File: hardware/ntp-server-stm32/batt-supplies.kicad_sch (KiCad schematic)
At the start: 24 parts, among them U34 TPS61094DSSR, U35 TPS61094DSSR

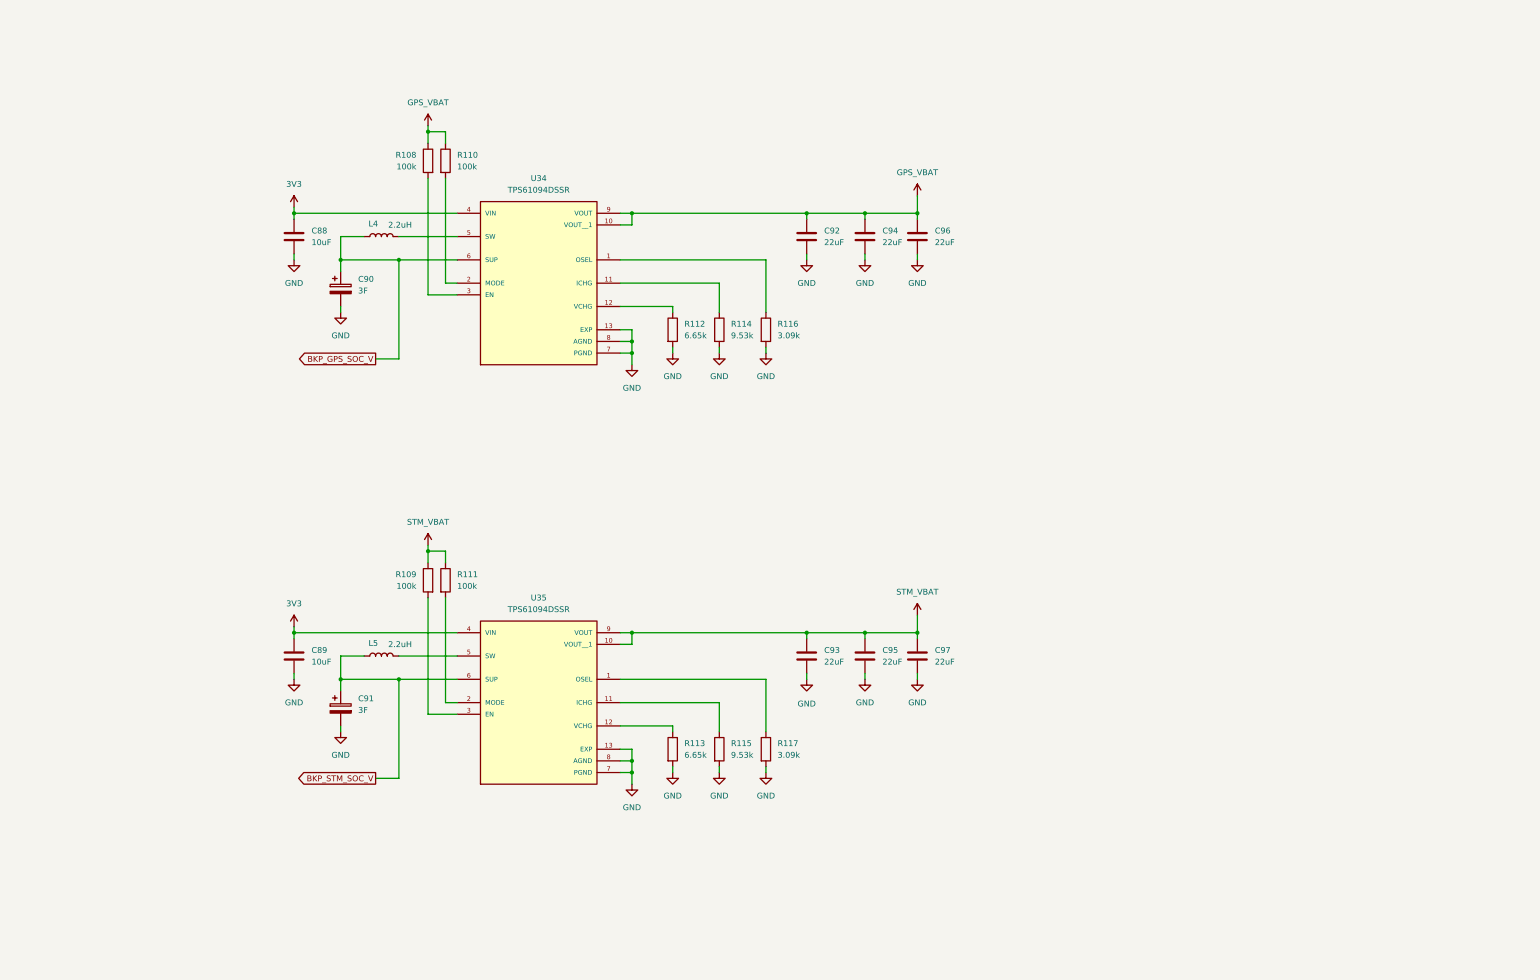
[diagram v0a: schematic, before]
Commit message: Updates
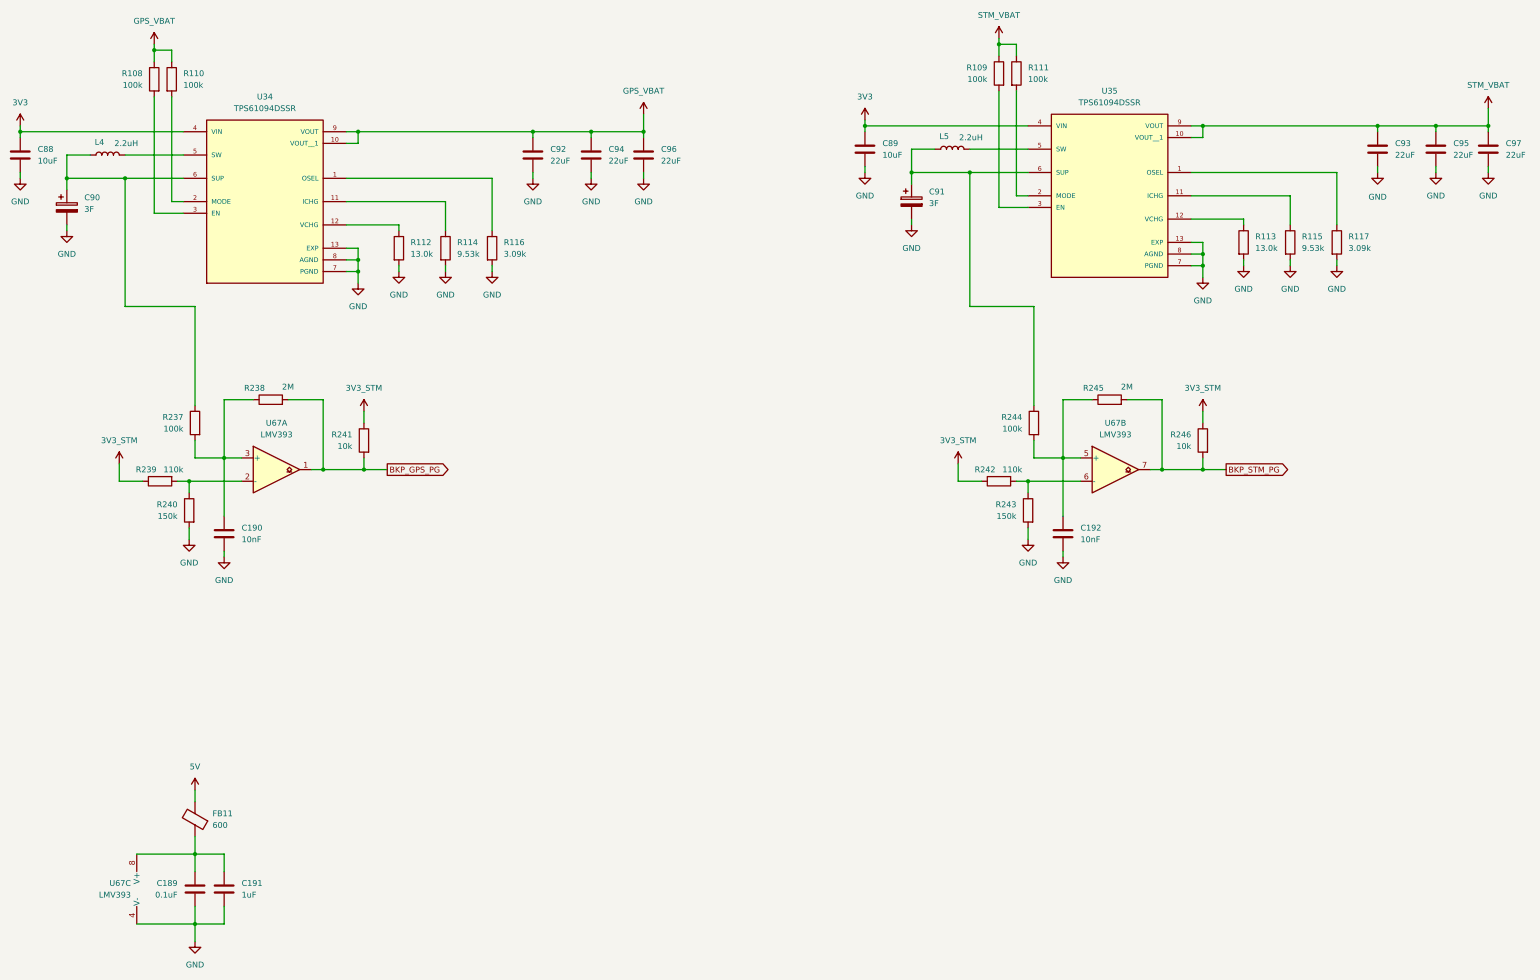
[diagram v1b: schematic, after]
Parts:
- added C189: 0.1uF, 0402 (1005 Metric), symbol Device:C
- added C190, C192: 10nF, 0402 (1005 Metric), symbol Device:C
- added C191: 1uF, 0603 (1608 Metric), symbol Device:C
- added FB11: 600, 1206, symbol Device:FerriteBead
- added R237, R244: 100k, 0402 (1005 Metric), symbol Device:R
- added R238, R245: 2M, 0402 (1005 Metric), symbol Device:R
- added R239, R242: 110k, R_0402_1005Metric, symbol Device:R
- added R240, R243: 150k, R_0402_1005Metric, symbol Device:R
- added R241, R246: 10k, 0402 (1005 Metric), symbol Device:R
- added U67: LMV393, symbol Comparator:LMV393
- C88, C89: footprint C_0805_2012Metric -> 1206 (3216 Metric); DIELECTRIC (none) -> X7R; DIGIKEY_PART_NUMBER 490-GRM21BZ71C106KE15LTR-ND -> 1276-6797-1-ND; MANUFACTURER Murata -> Samsung Electro-Mechanics; MANUFACTURER_PART_NUMBER GRM21BZ71C106KE15L -> CL31B106KOHVPNE; TOLERANCE (none) -> 10%; VOLTAGE (none) -> 16V
- C90, C91: DIELECTRIC (none) -> EDLC; MANUFACTURER Cornell Dubilier Knowles -> Cornell Dubilier; TOLERANCE (none) -> 5%; VOLTAGE (none) -> 3V
- C92, C93, C94, C95, C96, C97: footprint C_0805_2012Metric -> 0805 (2012 Metric); DIELECTRIC (none) -> X5R; DIGIKEY_PART_NUMBER (none) -> 490-GRT21BR61C226ME13KCT-ND; MANUFACTURER (none) -> Murata Electronics; MANUFACTURER_PART_NUMBER (none) -> GRT21BR61C226ME13K; TOLERANCE (none) -> 10%; VOLTAGE (none) -> 16V
- L4, L5: DIELECTRIC (none) -> Inductor
- R108, R109, R110, R111: footprint R_0402_1005Metric -> 0402 (1005 Metric); DIELECTRIC (none) -> Thick-film; DIGIKEY_PART_NUMBER (none) -> P100KLCT-ND; MANUFACTURER Panasonic -> Panasonic Industry; POWER (none) -> 1/10W; TOLERANCE (none) -> 1%
- R112, R113: value 6.65k -> 13.0k; footprint R_0402_1005Metric -> 0402 (1005 Metric); DIELECTRIC (none) -> Thick-film; DIGIKEY_PART_NUMBER (none) -> P13.0KLCT-ND; MANUFACTURER Panasonic -> Panasonic Industry; MANUFACTURER_PART_NUMBER ERJ-2RKF6651X -> ERJ-2RKF1302X; POWER (none) -> 1/10W; TOLERANCE (none) -> 1%
- R114, R115: footprint R_0402_1005Metric -> 0402 (1005 Metric); DIELECTRIC (none) -> Thick-film; DIGIKEY_PART_NUMBER (none) -> P9.53KLCT-ND; MANUFACTURER Panasonic -> Panasonic Industry; POWER (none) -> 1/10W; TOLERANCE (none) -> 1%
- R116, R117: footprint R_0402_1005Metric -> 0402 (1005 Metric); DIELECTRIC (none) -> Thick-film; DIGIKEY_PART_NUMBER (none) -> P3.09KLCT-ND; MANUFACTURER Panasonic -> Panasonic Industry; POWER (none) -> 1/10W; TOLERANCE (none) -> 1%
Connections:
- net GND: now also C189.2, C190.2, C191.2, C192.2, R240.2, R243.2, U67.4 (V-)
- net BKP_GPS_SOC_V: no longer names the net of C90.1, L4.2, U34.6 (SUP)
- net BKP_GPS_SOC_V: now also R237.1
- net BKP_STM_SOC_V: no longer names the net of C91.1, L5.2, U35.6 (SUP)
- net BKP_STM_SOC_V: now also R244.1
- new net: C190.1, R237.2, R238.1, U67.3 (+)
- new net: R239.2, R240.1, U67.2 (-)
- new net: R242.2, R243.1, U67.6 (-)
- new net: C192.1, R244.2, R245.1, U67.5 (+)
- new net: C189.1, C191.1, FB11.1, U67.8 (V+)
- new net 3V3_STM: R239.1, R241.1, R242.1, R246.1
- new net 5V: FB11.2
- new net BKP_GPS_PG: R238.2, R241.2, U67.1
- new net BKP_STM_PG: R245.2, R246.2, U67.7
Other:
- moved on the sheet: C88, C89, C90, C91, C92, C93, C94, C95, C96, C97, L4, L5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

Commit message: Bom updates
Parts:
- FB11: footprint 1206 -> 1206 (3216 Metric)
- L4, L5: DIGIKEY_PART_NUMBER (none) -> 283-DR73-2R2-RTR-ND; MANUFACTURER (none) -> Eaton - Electronics Division; MANUFACTURER_PART_NUMBER (none) -> DR73-2R2-R
- R239, R242: footprint R_0402_1005Metric -> 0402 (1005 Metric); DIGIKEY_PART_NUMBER (none) -> P110KLCT-ND; MANUFACTURER Panasonic -> Panasonic Industry
- R240, R243: footprint R_0402_1005Metric -> 0402 (1005 Metric); DIGIKEY_PART_NUMBER (none) -> P150KLCT-ND; MANUFACTURER Panasonic -> Panasonic Industry
- U34, U35: DIGIKEY_PART_NUMBER (none) -> 296-TPS61094DSSRCT-ND
- U67: footprint (none) -> 8-VSSOP; DIGIKEY_PART_NUMBER (none) -> 296-13993-1-ND
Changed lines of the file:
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@@
 			)
 		)
-		(property "Footprint" "R_0402_1005Metric"
+		(property "Footprint" "0402 (1005 Metric)"
 			(at 69.85 126.492 90)
 			(hide yes)
@@
 			)
 		)
-		(property "Datasheet" ""
+		(property "Datasheet" "https://industrial.panasonic.com/cdbs/www-data/pdf/RDA0000/AOA0000C304.pdf"
 			(at 69.85 128.27 0)
 			(hide yes)
@@
 			)
 		)
-		(property "Description" "RES 110k 1% 1/10W 0402"
+		(property "Description" "RES SMD 110K OHM 1% 1/10W 0402"
 			(at 69.85 128.27 0)
 			(hide yes)
@@
 			)
 		)
-		(property "MANUFACTURER" "Panasonic"
+		(property "MANUFACTURER" "Panasonic Industry"
 			(at 11.43 256.54 0)
 			(hide yes)
@@
 			)
 		)
+		(property "DIGIKEY_PART_NUMBER" "P110KLCT-ND"
+			(at 69.85 128.27 90)
+			(hide yes)
+			(show_name no)
+			(do_not_autoplace no)
+			(effects
+				(font
+					(size 1.27 1.27)
+				)
+			)
+		)
 		(pin "1"
 		)
@@
 			)
 		)
-		(property "Datasheet" ""
+		(property "Datasheet" "https://www.ti.com/general/docs/suppproductinfo.tsp?distId=10&gotoUrl=http%3A%2F%2Fwww.ti.com%2Flit%2Fgpn%2Ftps61094"
 			(at 92.71 67.31 0)
 			(hide yes)
@@
 			)
 		)
+		(property "DIGIKEY_PART_NUMBER" "296-TPS61094DSSRCT-ND"
+			(at 92.71 67.31 0)
+			(hide yes)
+			(show_name no)
+			(do_not_autoplace no)
+			(effects
+				(font
+					(size 1.27 1.27)
+				)
+			)
+		)
 		(pin "13"
 		)
@@
 			)
 		)
-		(property "Footprint" "R_0402_1005Metric"
+		(property "Footprint" "0402 (1005 Metric)"
 			(at 260.858 134.62 90)
 			(hide yes)
@@
 			)
 		)
-		(property "Datasheet" ""
+		(property "Datasheet" "https://industrial.panasonic.com/cdbs/www-data/pdf/RDA0000/AOA0000C304.pdf"
 			(at 259.08 134.62 0)
 			(hide yes)
@@
 			)
 		)
-		(property "Description" "RES 150k 1% 1/10W 0402"
+		(property "Description" "RES SMD 150K OHM 1% 1/10W 0402"
 			(at 259.08 134.62 0)
 			(hide yes)
@@
 			)
 		)
-		(property "MANUFACTURER" "Panasonic"
+		(property "MANUFACTURER" "Panasonic Industry"
 			(at 130.81 76.2 0)
 			(hide yes)
@@
 			)
 		)
+		(property "DIGIKEY_PART_NUMBER" "P150KLCT-ND"
+			(at 259.08 134.62 0)
+			(hide yes)
+			(show_name no)
+			(do_not_autoplace no)
+			(effects
+				(font
+					(size 1.27 1.27)
+				)
+			)
+		)
 		(pin "1"
 		)
@@
 			)
 		)
-		(property "Datasheet" ""
+		(property "Datasheet" "https://www.ti.com/general/docs/suppproductinfo.tsp?distId=10&gotoUrl=http%3A%2F%2Fwww.ti.com%2Flit%2Fgpn%2Ftps61094"
 			(at 276.86 66.04 0)
 			(hide yes)
@@
 			)
 		)
+		(property "DIGIKEY_PART_NUMBER" "296-TPS61094DSSRCT-ND"
+			(at 276.86 66.04 0)
+			(hide yes)
+			(show_name no)
+			(do_not_autoplace no)
+			(effects
+				(font
+					(size 1.27 1.27)
+				)
+			)
+		)
 		(pin "13"
 		)
@@
 			)
 		)
-		(property "Footprint" "R_0402_1005Metric"
+		(property "Footprint" "0402 (1005 Metric)"
 			(at 252.73 126.492 90)
 			(hide yes)
@@
 			)
 		)
-		(property "Datasheet" ""
+		(property "Datasheet" "https://industrial.panasonic.com/cdbs/www-data/pdf/RDA0000/AOA0000C304.pdf"
 			(at 252.73 128.27 0)
 			(hide yes)
@@
 			)
 		)
-		(property "Description" "RES 110k 1% 1/10W 0402"
+		(property "Description" "RES SMD 110K OHM 1% 1/10W 0402"
 			(at 252.73 128.27 0)
 			(hide yes)
@@
 			)
 		)
-		(property "MANUFACTURER" "Panasonic"
+		(property "MANUFACTURER" "Panasonic Industry"
 			(at 194.31 256.54 0)
 			(hide yes)
@@
 			)
 		)
+		(property "DIGIKEY_PART_NUMBER" "P110KLCT-ND"
+			(at 252.73 128.27 90)
+			(hide yes)
+			(show_name no)
+			(do_not_autoplace no)
+			(effects
+				(font
+					(size 1.27 1.27)
+				)
+			)
+		)
 		(pin "1"
 		)
@@
 			)
 		)
-		(property "Datasheet" ""
+		(property "Datasheet" "https://www.eaton.com/content/dam/eaton/products/electronic-components/resources/data-sheet/eaton-dr-high-power-density-high-efficiency-shielded-drum-core-power-inductors-data-sheet.pdf"
 			(at 58.42 57.15 0)
 			(hide yes)
@@
 			)
 		)
-		(property "Description" "IND 2.2uH"
+		(property "Description" "IND 2.2uH 4.15A"
 			(at 58.42 57.15 0)
 			(hide yes)
@@
 			)
 		)
+		(property "DIGIKEY_PART_NUMBER" "283-DR73-2R2-RTR-ND"
+			(at 58.42 57.15 90)
+			(hide yes)
+			(show_name no)
+			(do_not_autoplace no)
+			(effects
+				(font
+					(size 1.27 1.27)
+				)
+			)
+		)
+		(property "MANUFACTURER" "Eaton - Electronics Division"
+			(at 58.42 57.15 90)
+			(hide yes)
+			(show_name no)
+			(do_not_autoplace no)
+			(effects
+				(font
+					(size 1.27 1.27)
+				)
+			)
+		)
+		(property "MANUFACTURER_PART_NUMBER" "DR73-2R2-R"
+			(at 58.42 57.15 90)
+			(hide yes)
+			(show_name no)
+			(do_not_autoplace no)
+			(effects
+				(font
+					(size 1.27 1.27)
+				)
+			)
+		)
 		(pin "1"
 		)
@@
 			)
 		)
-		(property "Footprint" ""
+		(property "Footprint" "8-VSSOP"
 			(at 95.25 125.73 0)
 			(hide yes)
@@
 			)
 		)
-		(property "Datasheet" "http://www.ti.com/lit/ds/symlink/lmv331.pdf"
+		(property "Datasheet" "https://www.ti.com/general/docs/suppproductinfo.tsp?distId=10&gotoUrl=https%3A%2F%2Fwww.ti.com%2Flit%2Fgpn%2Flmv393"
 			(at 95.25 125.73 0)
 			(hide yes)
@@
 			)
 		)
-		(property "Description" "Dual comparator low-voltage"
+		(property "Description" "IC COMPARATOR 2CH 8-VSSOP"
 			(at 95.25 125.73 0)
 			(hide yes)
@@
 			)
 		)
+		(property "DIGIKEY_PART_NUMBER" "296-13993-1-ND"
+			(at 95.25 125.73 0)
+			(hide yes)
+			(show_name no)
+			(do_not_autoplace no)
+			(effects
+				(font
+					(size 1.27 1.27)
+				)
+			)
+		)
 		(pin "3"
 		)
@@
 			)
 		)
-		(property "Footprint" ""
+		(property "Footprint" "8-VSSOP"
 			(at 278.13 125.73 0)
 			(hide yes)
@@
 			)
 		)
-		(property "Datasheet" "http://www.ti.com/lit/ds/symlink/lmv331.pdf"
+		(property "Datasheet" "https://www.ti.com/general/docs/suppproductinfo.tsp?distId=10&gotoUrl=https%3A%2F%2Fwww.ti.com%2Flit%2Fgpn%2Flmv393"
 			(at 278.13 125.73 0)
 			(hide yes)
@@
 			)
 		)
-		(property "Description" "Dual comparator low-voltage"
+		(property "Description" "IC COMPARATOR 2CH 8-VSSOP"
 			(at 278.13 125.73 0)
 			(hide yes)
@@
 			)
 		)
+		(property "DIGIKEY_PART_NUMBER" "296-13993-1-ND"
+			(at 278.13 125.73 0)
+			(hide yes)
+			(show_name no)
+			(do_not_autoplace no)
+			(effects
+				(font
+					(size 1.27 1.27)
+				)
+			)
+		)
 		(pin "3"
 		)
@@
 			)
 		)
-		(property "Footprint" ""
+		(property "Footprint" "8-VSSOP"
 			(at 62.23 217.17 0)
 			(hide yes)
@@
 			)
 		)
-		(property "Datasheet" "http://www.ti.com/lit/ds/symlink/lmv331.pdf"
+		(property "Datasheet" "https://www.ti.com/general/docs/suppproductinfo.tsp?distId=10&gotoUrl=https%3A%2F%2Fwww.ti.com%2Flit%2Fgpn%2Flmv393"
 			(at 62.23 217.17 0)
 			(hide yes)
@@
 			)
 		)
-		(property "Description" "Dual comparator low-voltage"
+		(property "Description" "IC COMPARATOR 2CH 8-VSSOP"
 			(at 62.23 217.17 0)
 			(hide yes)
@@
 			)
 		)
+		(property "DIGIKEY_PART_NUMBER" "296-13993-1-ND"
+			(at 62.23 217.17 0)
+			(hide yes)
+			(show_name no)
+			(do_not_autoplace no)
+			(effects
+				(font
+					(size 1.27 1.27)
+				)
+			)
+		)
 		(pin "3"
 		)
@@
 			)
 		)
-		(property "Datasheet" ""
+		(property "Datasheet" "https://www.eaton.com/content/dam/eaton/products/electronic-components/resources/data-sheet/eaton-dr-high-power-density-high-efficiency-shielded-drum-core-power-inductors-data-sheet.pdf"
 			(at 242.57 55.88 0)
 			(hide yes)
@@
 			)
 		)
-		(property "Description" "IND 2.2uH"
+		(property "Description" "IND 2.2uH 4.15A"
 			(at 242.57 55.88 0)
 			(hide yes)
@@
 			)
 		)
+		(property "DIGIKEY_PART_NUMBER" "283-DR73-2R2-RTR-ND"
+			(at 242.57 55.88 90)
+			(hide yes)
+			(show_name no)
+			(do_not_autoplace no)
+			(effects
+				(font
+					(size 1.27 1.27)
+				)
+			)
+		)
+		(property "MANUFACTURER" "Eaton - Electronics Division"
+			(at 242.57 55.88 90)
+			(hide yes)
+			(show_name no)
+			(do_not_autoplace no)
+			(effects
+				(font
+					(size 1.27 1.27)
+				)
+			)
+		)
+		(property "MANUFACTURER_PART_NUMBER" "DR73-2R2-R"
+			(at 242.57 55.88 90)
+			(hide yes)
+			(show_name no)
+			(do_not_autoplace no)
+			(effects
+				(font
+					(size 1.27 1.27)
+				)
+			)
+		)
 		(pin "1"
 		)
@@
 			)
 		)
-		(property "Footprint" "R_0402_1005Metric"
+		(property "Footprint" "0402 (1005 Metric)"
 			(at 77.978 134.62 90)
 			(hide yes)
@@
 			)
 		)
-		(property "Datasheet" ""
+		(property "Datasheet" "https://industrial.panasonic.com/cdbs/www-data/pdf/RDA0000/AOA0000C304.pdf"
 			(at 76.2 134.62 0)
 			(hide yes)
@@
 			)
 		)
-		(property "Description" "RES 150k 1% 1/10W 0402"
+		(property "Description" "RES SMD 150K OHM 1% 1/10W 0402"
 			(at 76.2 134.62 0)
 			(hide yes)
@@
 			)
 		)
-		(property "MANUFACTURER" "Panasonic"
+		(property "MANUFACTURER" "Panasonic Industry"
 			(at -52.07 76.2 0)
 			(hide yes)
@@
 			)
 		)
+		(property "DIGIKEY_PART_NUMBER" "P150KLCT-ND"
+			(at 76.2 134.62 0)
+			(hide yes)
+			(show_name no)
+			(do_not_autoplace no)
+			(effects
+				(font
+					(size 1.27 1.27)
+				)
+			)
+		)
 		(pin "1"
 		)
@@
 			)
 		)
-		(property "Footprint" "1206"
+		(property "Footprint" "1206 (3216 Metric)"
 			(at 79.248 201.93 90)
 			(hide yes)
